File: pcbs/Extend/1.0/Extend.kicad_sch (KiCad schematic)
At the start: 24 parts, among them J1 Conn_01x06_Pin, J10 Conn_01x02_Male, J13 Conn_01x04_Pin, J2 Conn_01x05_Pin, J3 Conn_01x04_Pin, J4 Conn_01x02_Male, J5 Conn_01x02_Male, J6 Conn_01x02_Male, J7 Conn_01x02_Pin, J8 Conn_01x05_Pin, J9 Conn_01x02_Pin, U1 MCP23017_SS

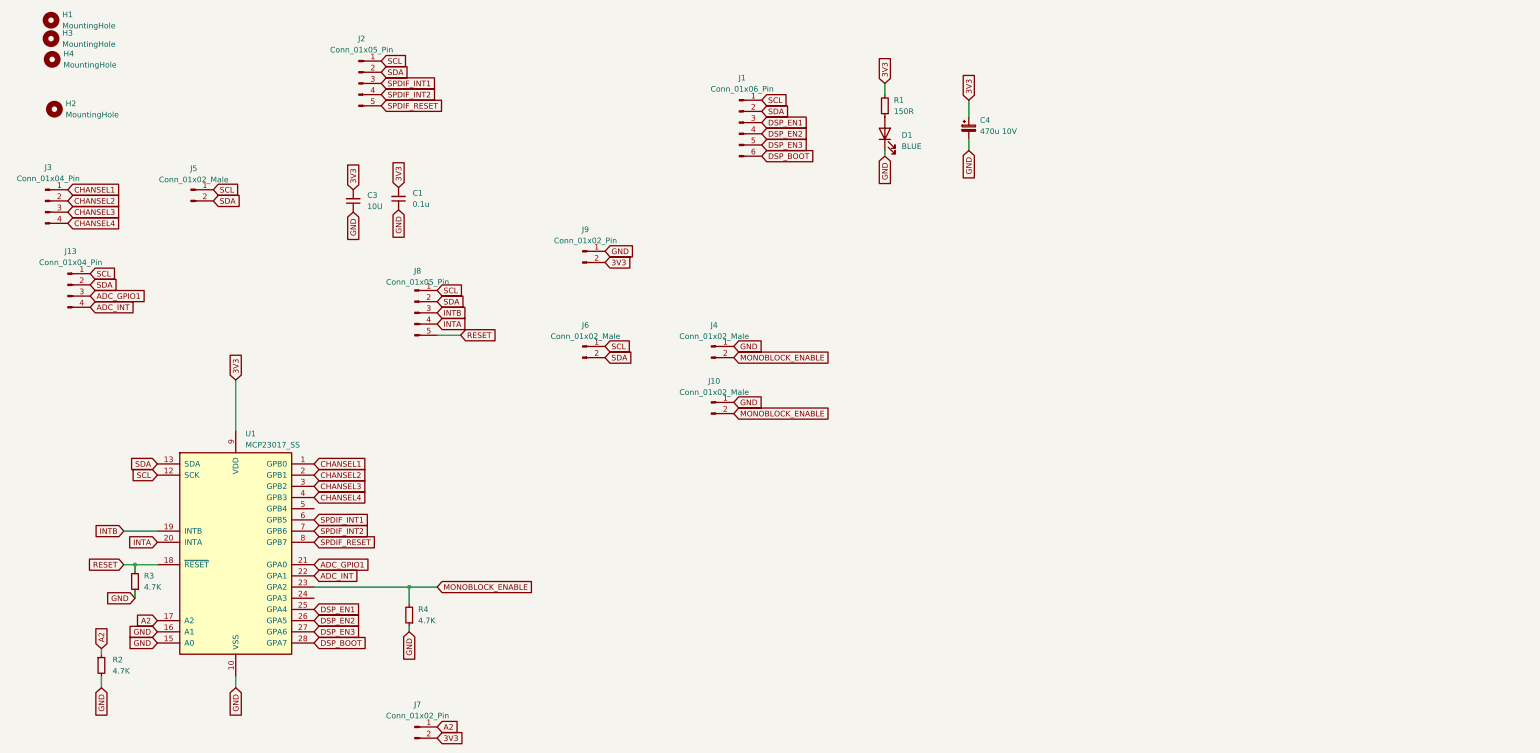
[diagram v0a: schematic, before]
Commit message: Updates
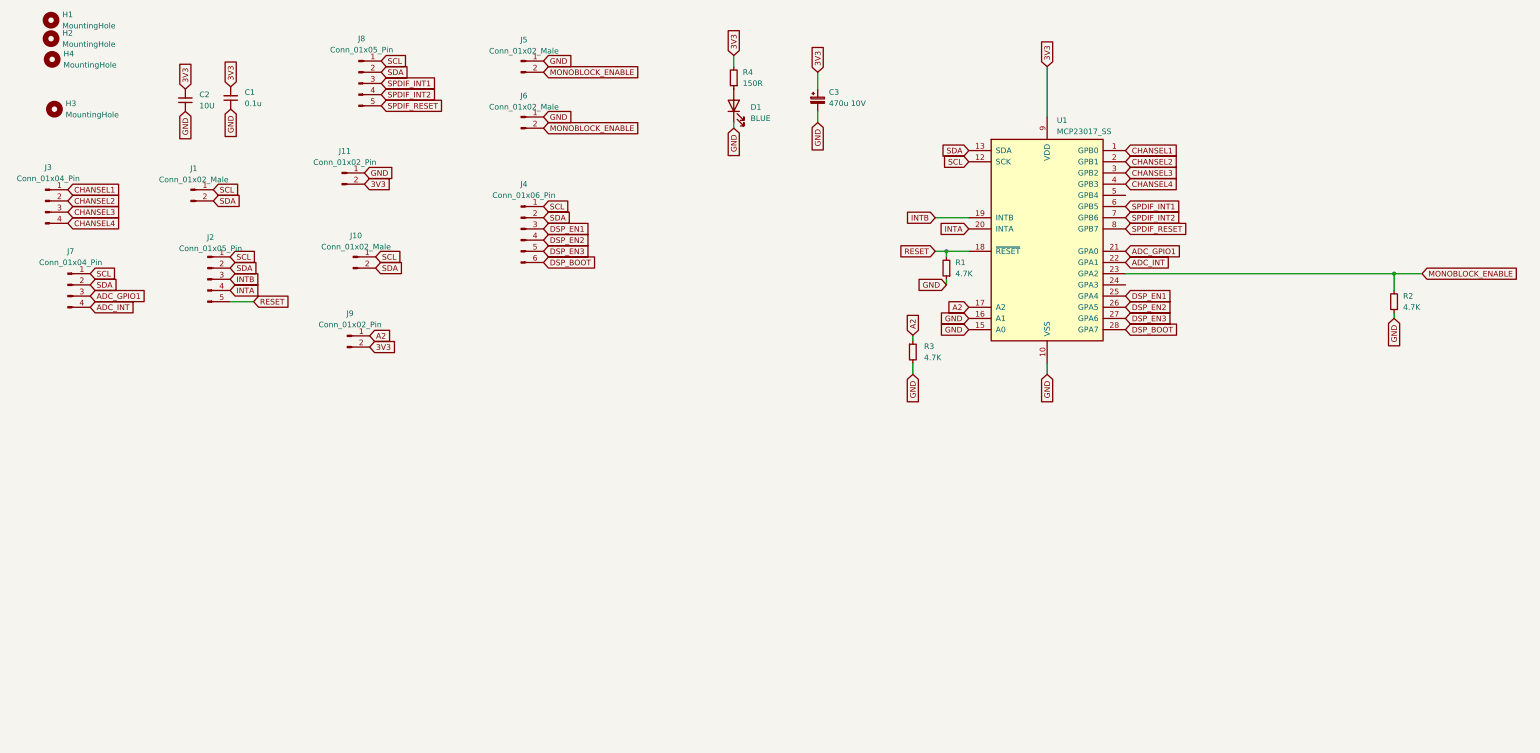
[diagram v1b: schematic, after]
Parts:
- renumbered C3 to C2, C4 to C3, H3 to H2, H2 to H3, J5 to J1, J6 to J10, J9 to J11, J8 to J2, J1 to J4, J4 to J5, J10 to J6, J13 to J7, J2 to J8, J7 to J9, R3 to R1, R4 to R2, R2 to R3, R1 to R4
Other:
- moved on the sheet: C1, C2, C3, D1, J10, J11, J2, J4, J5, J6, J9, R1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
